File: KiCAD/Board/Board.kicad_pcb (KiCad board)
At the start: 4 copper layers, 59.9 x 50.4 mm, 64 parts, among them J1 USB_OTG, J2 JST_BATT, J4 Conn_Coaxial, J5 Conn_02x05_Odd_Even, Q1 PWR_PMOS, SW1 ON_OFF, U1 MCP73831-2-OT, U2 USBLC6-2SC6, U3 ME6211A28M3G-N, U4 DS-32-BLE4.2, U5 STM32L151C8TxA, U6 ATGM336H-1N, U7 MPU-6050, U8 Micro_SD_TF-15, U9 MLX90393

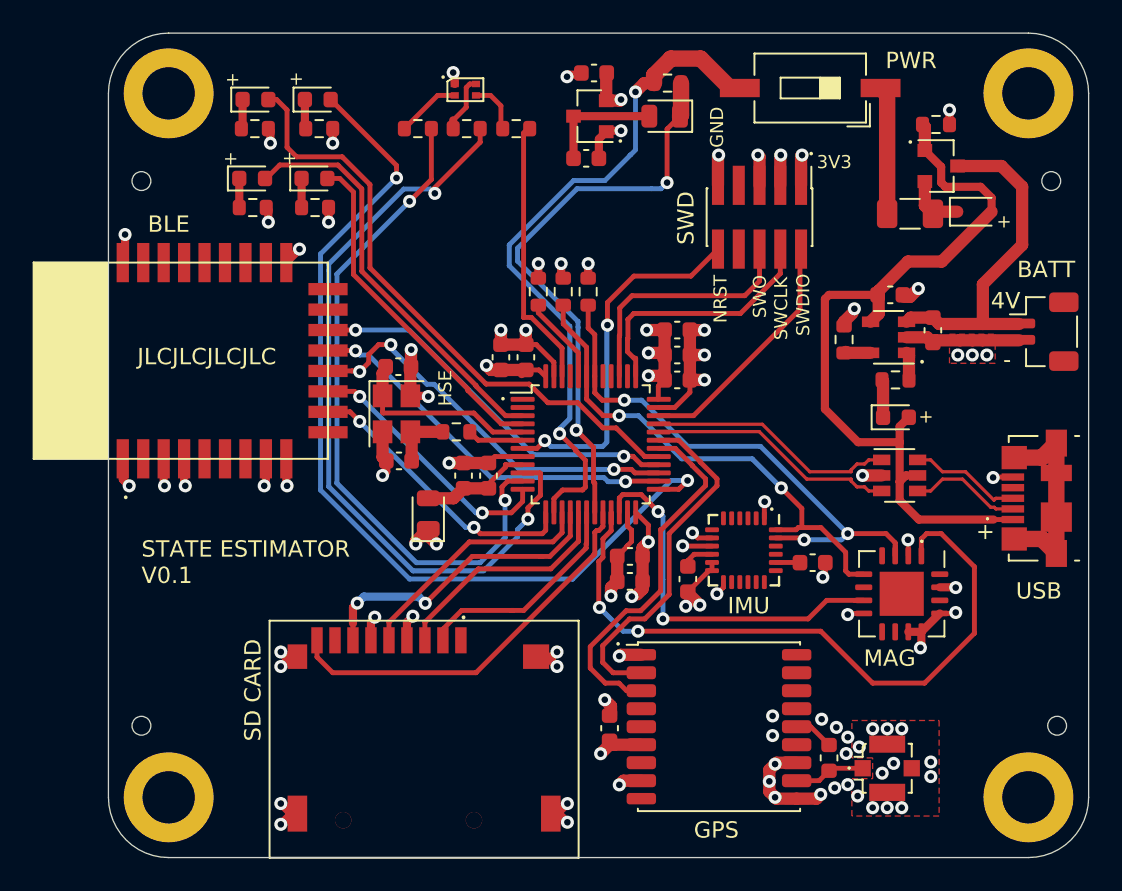
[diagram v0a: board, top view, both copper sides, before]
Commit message: submitted board to JLCPCB
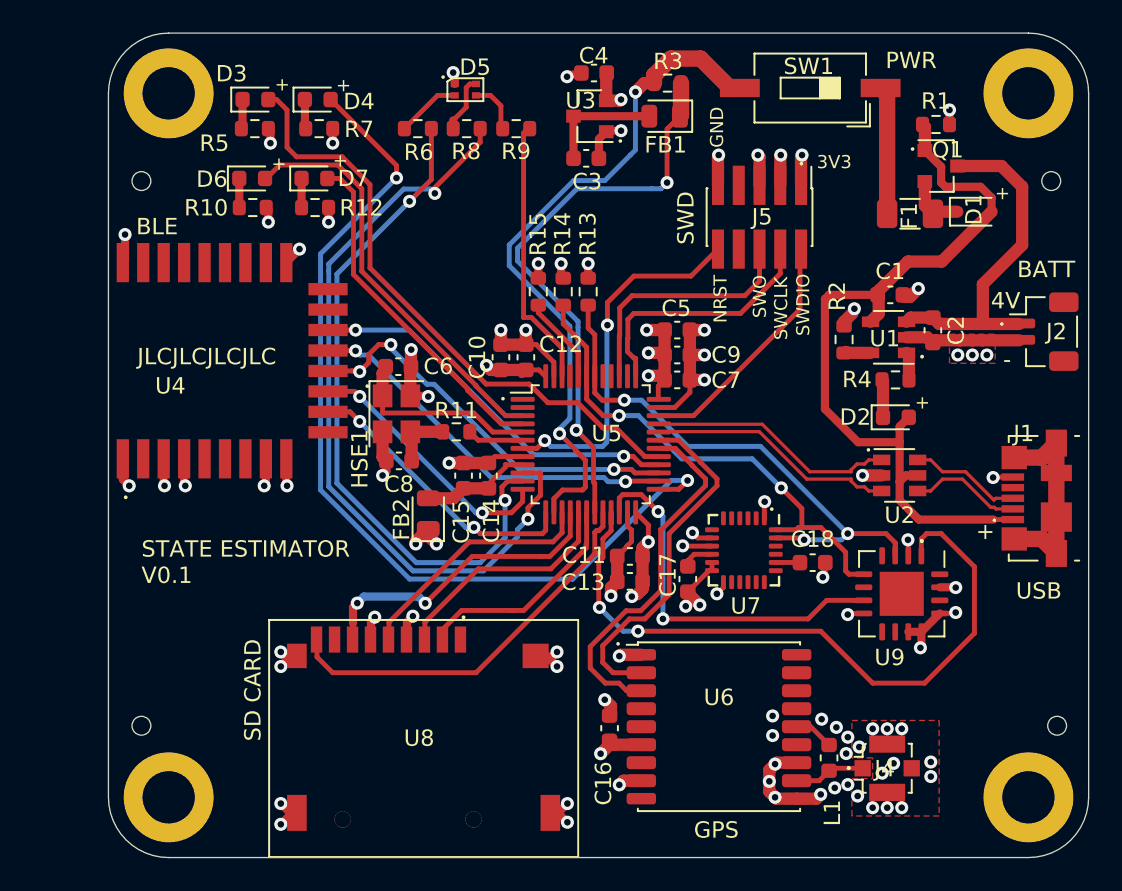
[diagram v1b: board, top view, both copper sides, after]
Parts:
- moved U8 0.05 mm to (137.3, 104.7)
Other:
- board text removed: "HSE"
- board text removed: "IMU"
- board text removed: "MAG"
